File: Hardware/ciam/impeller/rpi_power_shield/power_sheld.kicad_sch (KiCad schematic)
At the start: 54 parts, among them J1 Micro-fit_1x2P, J12 Micro-Fit_2x2P, J2 RPi, J3 Micro-fit_1x2P, K1 NRP-12-C-05D-H, Q1 BSS138, Q5 BSS138, U2 L4940V5, U3 VDV8-1E05, U4 B0505MT-1WR4, U46 HCPL-0600

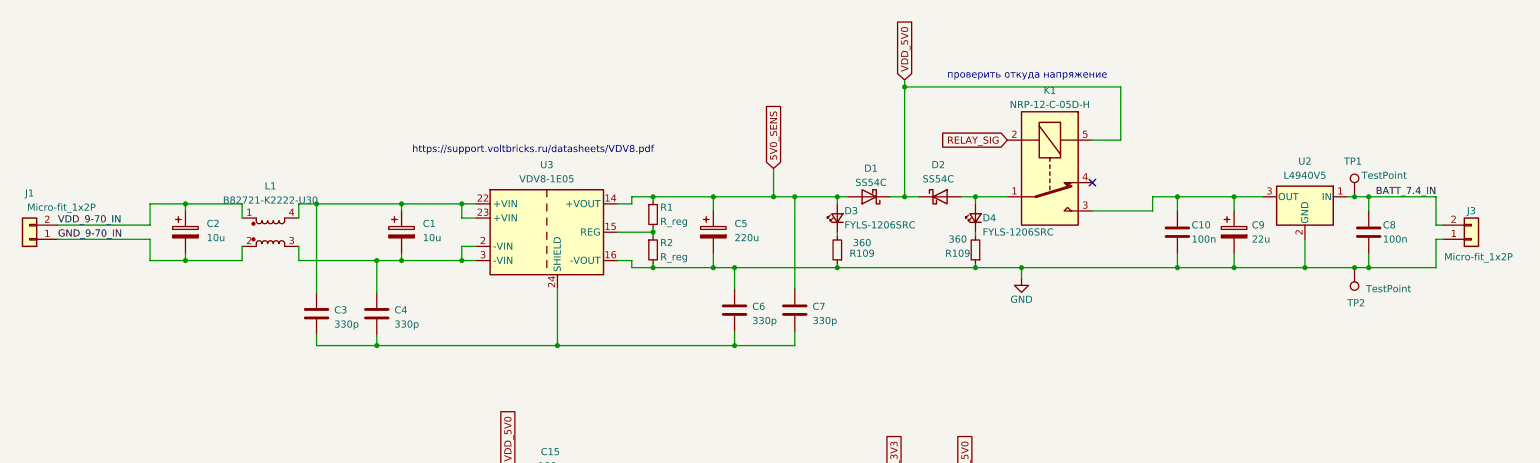
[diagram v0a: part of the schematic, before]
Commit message: Updated CIAM project
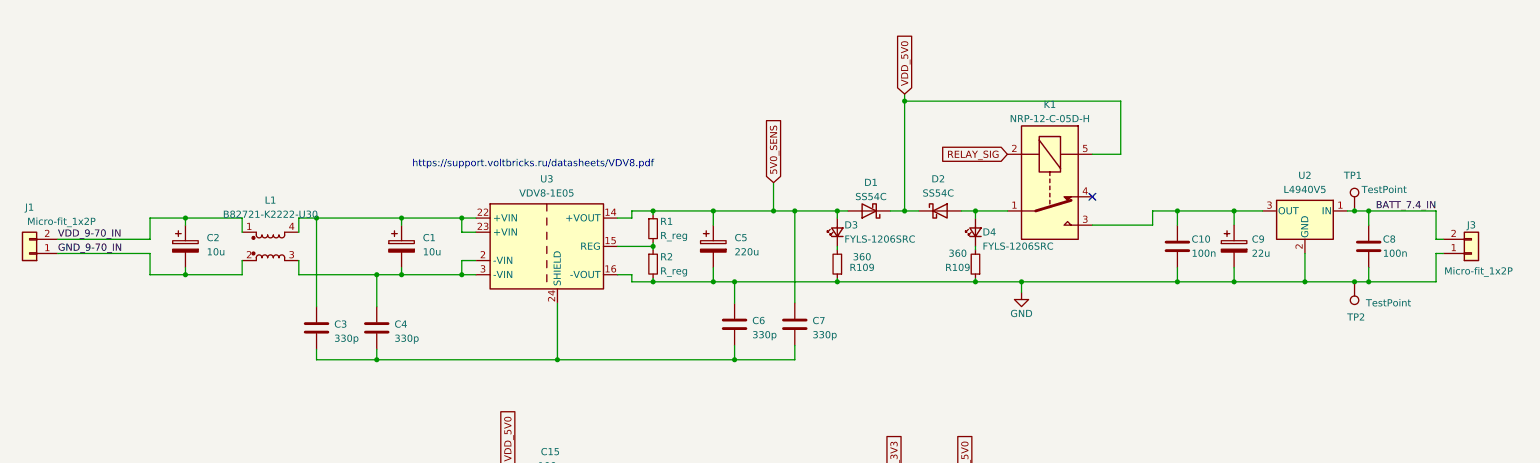
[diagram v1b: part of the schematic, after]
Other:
- note removed: "проверить откуда напряжение"
- moved on the sheet: C1, C10, C2, C3, C4, C5, C6, C7, C8, C9, D1, D2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
